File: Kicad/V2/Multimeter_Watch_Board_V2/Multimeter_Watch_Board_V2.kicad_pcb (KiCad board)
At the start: 4 copper layers, 46 x 42 mm, 61 parts, among them J1 S3B-PH-K-S(LF)(SN), J2 S3B-PH-K-S(LF)(SN), J3 S3B-PH-K-S(LF)(SN), J6 51281-1294, J7 Conn_01x11_Female, J8 Conn_01x11_Female, Q1 A03400A N-MOS, U1 PCF85163-SO08, U2 AD8592, Y1 32kHz

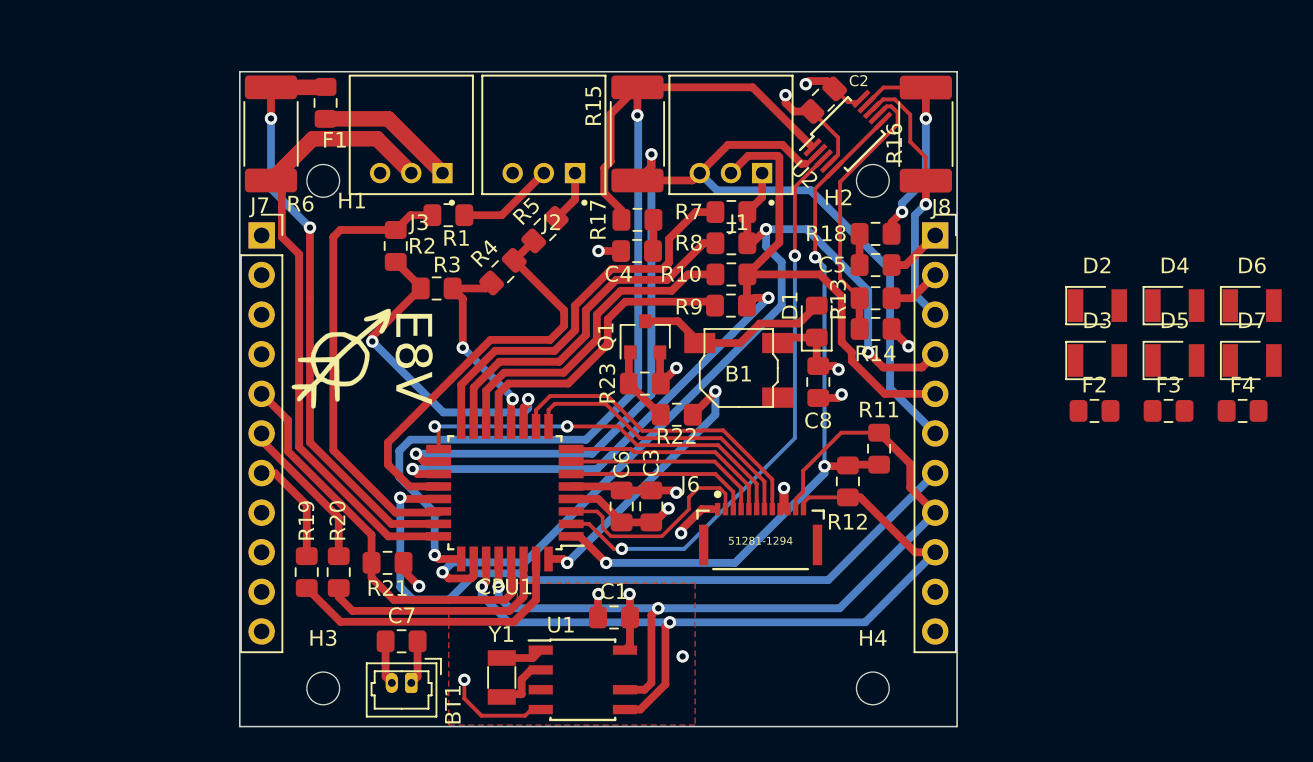
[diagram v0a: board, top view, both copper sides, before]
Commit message: implement rlc protection (likely to be reverted)
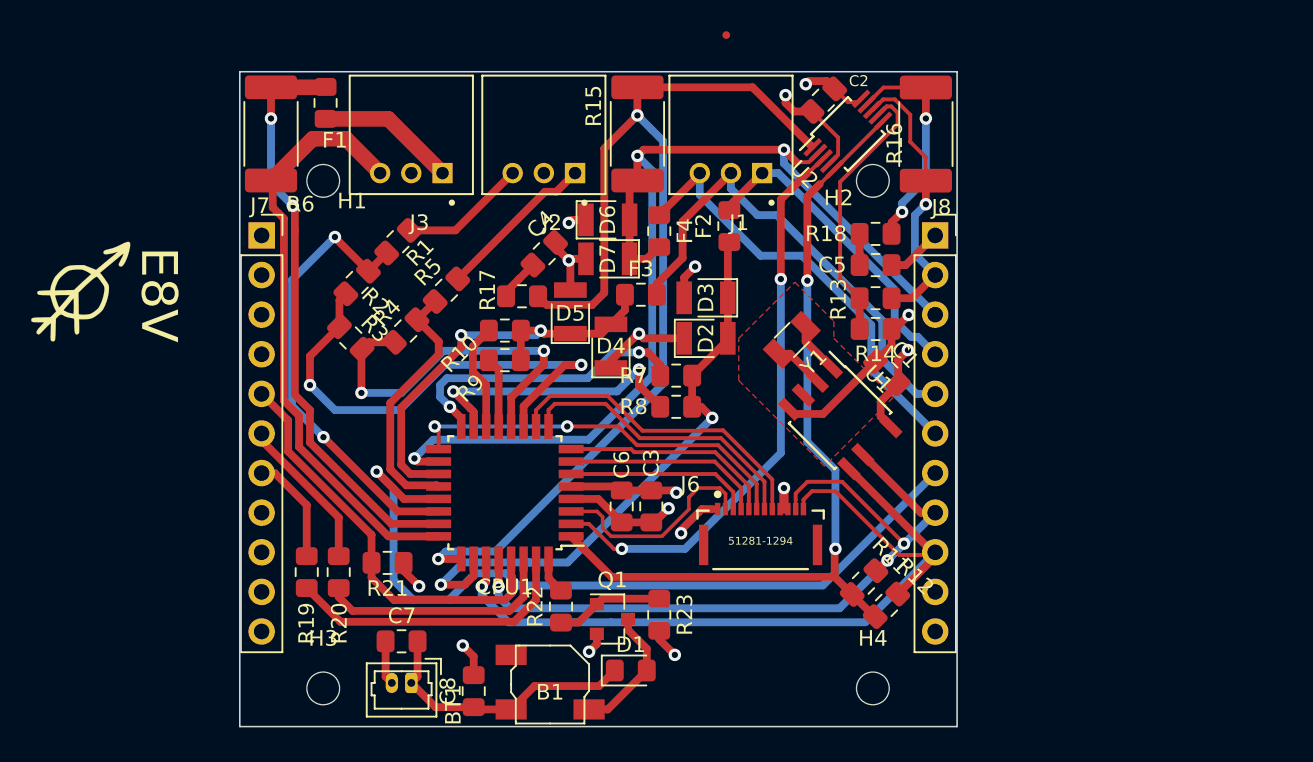
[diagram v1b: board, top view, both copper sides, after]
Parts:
- moved D7 41.8 mm to (125.6, 70.0), turned to 180 degrees
- moved D6 41.7 mm to (125.6, 67.5)
- moved F4 39.2 mm to (128.9, 68.2), turned to 270 degrees
- moved D5 38.9 mm to (123.2, 73.4), turned to 90 degrees
- moved D4 36.3 mm to (125.8, 75.6), turned to 90 degrees
- moved F3 34.7 mm to (127.7, 72.3)
- moved C8 29.7 mm to (117.0, 97.7), turned to 90 degrees
- moved Y1 28.5 mm to (137.4, 75.2), turned to 225 degrees
- moved F2 26.2 mm to (133.4, 67.9), turned to 90 degrees
- moved D3 25.4 mm to (131.9, 72.5), turned to 180 degrees
- moved D1 25.4 mm to (127.1, 96.4), turned to 0 degrees
- moved D2 25.2 mm to (131.9, 75.1)
- moved B1 23.6 mm to (121.9, 97.3), turned to 0 degrees
- moved U1 23.5 mm to (140.5, 80.2), turned to 315 degrees
- moved C1 23.5 mm to (143.5, 77.3), turned to 315 degrees
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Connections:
- F2 pad 2: Net-(F2-Pad2) -> /RLC1
- F3 pad 2: Net-(F3-Pad2) -> /RLC2
- F4 pad 1: Net-(F4-Pad1) -> /RLC3
- J1 pad 1: Net-(F2-Pad2) -> /RLC1
- J1 pad 2: Net-(F3-Pad2) -> /RLC2
- J1 pad 3: Net-(F4-Pad1) -> /RLC3
- J3 pad 2: /ADC1 -> Net-(J3-Pad2)
- J3 pad 3: Net-(J3-Pad3) -> /ADC1
- J8 pad 2: /VCC -> /VCC_HALF
- J8 pad 3: /VCC_HALF -> /DACout
- J8 pad 4: /ADC3 -> /RLC1
- J8 pad 5: /ADC6 -> /RLC2
- J8 pad 6: /DACout -> /RLC3
- R1 pad 1: Net-(J2-Pad2) -> Net-(J2-Pad3)
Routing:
- net /ADC6: track 62.0 -> 28.3 mm
- net /RLC2: track 0.00 -> 30.8 mm
- net /RLC3: track 0.00 -> 28.4 mm
- net /ADC3: track 61.2 -> 38.6 mm, vias 3 -> 2
- net /RLC1: track 0.00 -> 20.3 mm
- net /VCC: track 32.5 -> 50.7 mm, vias 6 -> 7
- net /PD2: track 18.3 -> 2.36 mm, vias 2 -> 0
- net /PB1: track 19.5 -> 4.51 mm
- net /PB2: track 21.0 -> 6.93 mm
- net /PD7: track 21.6 -> 32.2 mm
- net /PB0: track 13.1 -> 23.6 mm
- net /ADC10: track 26.9 -> 16.7 mm
- net Net-(J2-Pad3): track 0.00 -> 8.16 mm
- net /DACout: track 76.9 -> 69.6 mm, vias 2 -> 3
- net /GND: track 38.2 -> 45.5 mm, vias 10 -> 9
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
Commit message: Revert "implement rlc protection (likely to be reverted)"
This reverts commit 3bbffdcc62f9ba327af4a0488dca8880d003efb7.
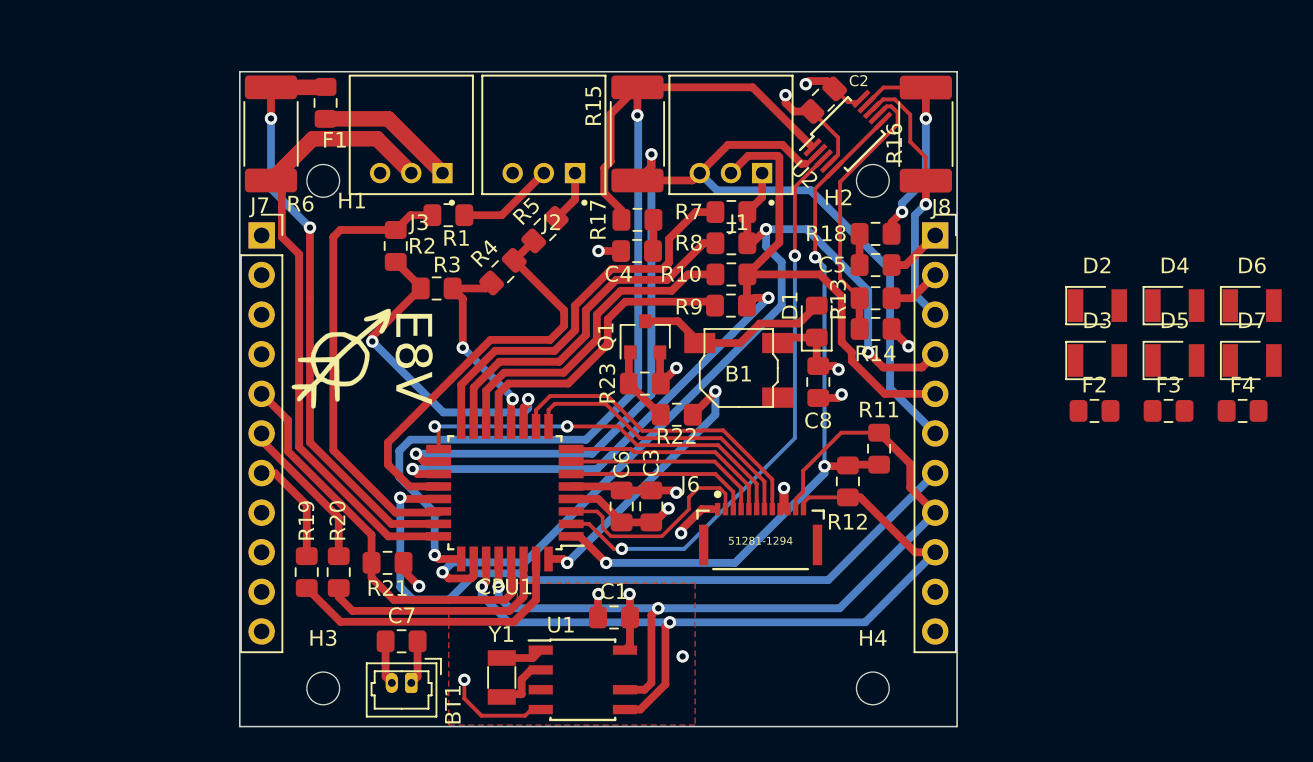
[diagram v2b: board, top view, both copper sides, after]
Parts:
- moved D7 41.8 mm to (166.9, 76.5), turned to 0 degrees
- moved D6 41.7 mm to (166.9, 73.0)
- moved F4 39.2 mm to (166.3, 79.8), turned to 0 degrees
- moved D5 38.9 mm to (162.0, 76.5), turned to 0 degrees
- moved D4 36.3 mm to (162.0, 73.0), turned to 0 degrees
- moved F3 34.7 mm to (161.6, 79.8)
- moved C8 29.7 mm to (139.1, 77.9), turned to 270 degrees
- moved Y1 28.5 mm to (118.8, 96.8), turned to 270 degrees
- moved F2 26.2 mm to (156.8, 79.8), turned to 0 degrees
- moved D3 25.4 mm to (157.0, 76.5), turned to 0 degrees
- moved D1 25.4 mm to (139.0, 74.0), turned to 90 degrees
- moved D2 25.2 mm to (157.0, 73.0)
- moved B1 23.6 mm to (134.0, 77.0), turned to 180 degrees
- moved U1 23.5 mm to (124.0, 97.0), turned to 0 degrees
- moved C1 23.5 mm to (126.0, 93.0), turned to 0 degrees
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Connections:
- F2 pad 2: /RLC1 -> Net-(F2-Pad2)
- F3 pad 2: /RLC2 -> Net-(F3-Pad2)
- F4 pad 1: /RLC3 -> Net-(F4-Pad1)
- J1 pad 1: /RLC1 -> Net-(F2-Pad2)
- J1 pad 2: /RLC2 -> Net-(F3-Pad2)
- J1 pad 3: /RLC3 -> Net-(F4-Pad1)
- J3 pad 2: Net-(J3-Pad2) -> /ADC1
- J3 pad 3: /ADC1 -> Net-(J3-Pad3)
- J8 pad 2: /VCC_HALF -> /VCC
- J8 pad 3: /DACout -> /VCC_HALF
- J8 pad 4: /RLC1 -> /ADC3
- J8 pad 5: /RLC2 -> /ADC6
- J8 pad 6: /RLC3 -> /DACout
- R1 pad 1: Net-(J2-Pad3) -> Net-(J2-Pad2)
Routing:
- net /ADC6: track 28.3 -> 62.0 mm
- net /RLC2: track 30.8 -> 0.00 mm
- net /RLC3: track 28.4 -> 0.00 mm
- net /ADC3: track 38.6 -> 61.2 mm, vias 2 -> 3
- net /RLC1: track 20.3 -> 0.00 mm
- net /VCC: track 50.7 -> 32.5 mm, vias 7 -> 6
- net /PD2: track 2.36 -> 18.3 mm, vias 0 -> 2
- net /PB1: track 4.51 -> 19.5 mm
- net /PB2: track 6.93 -> 21.0 mm
- net /PD7: track 32.2 -> 21.6 mm
- net /PB0: track 23.6 -> 13.1 mm
- net /ADC10: track 16.7 -> 26.9 mm
- net Net-(J2-Pad3): track 8.16 -> 0.00 mm
- net /DACout: track 69.6 -> 76.9 mm, vias 3 -> 2
- net /GND: track 45.5 -> 38.2 mm, vias 9 -> 10
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
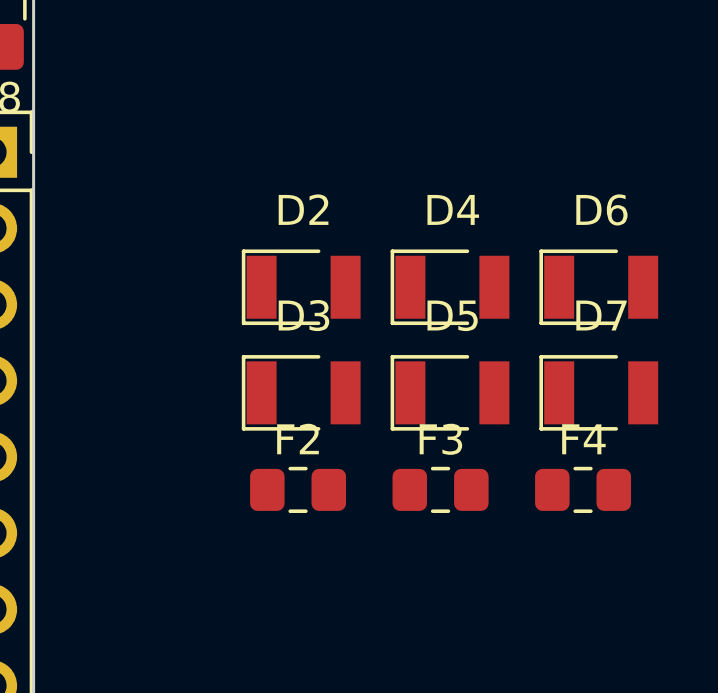
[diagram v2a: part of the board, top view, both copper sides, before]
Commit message: Revert "add rlc tester protection to schematic"
This reverts commit df46bc8d5560e11f4e55d6f466ca62c966db9fe4.
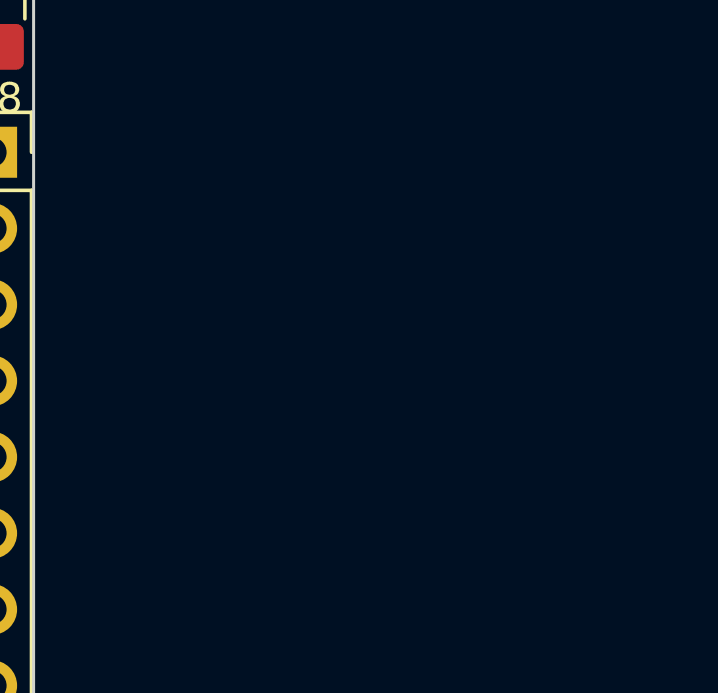
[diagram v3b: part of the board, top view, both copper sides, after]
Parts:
- removed D2, D3, D4, D5, D6, D7: D, Multimeter_Watch_Custom_Footprints:1408D
- removed F2, F3, F4: Fuse, Fuse:Fuse_0805_2012Metric_Pad1.15x1.40mm_HandSolder
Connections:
- J1 pad 1: Net-(F2-Pad2) -> /ADC3
- J1 pad 2: Net-(F3-Pad2) -> /ADC6
- J1 pad 3: Net-(F4-Pad1) -> /DACout
- R19 pad 1: /D1 -> Net-(CPU1-Pad31)
- R19 pad 2: Net-(CPU1-Pad31) -> /D1
- R20 pad 1: /D0 -> Net-(CPU1-Pad30)
- R20 pad 2: Net-(CPU1-Pad30) -> /D0
